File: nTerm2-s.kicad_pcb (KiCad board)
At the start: 2 copper layers, 147.3 x 55.9 mm, 107 parts, among them J1 VGA, J2 Keyboard, J3 Mouse, J4 Speaker, J5 DE9_Plug_MountingHoles, J6 USB_C_Receptacle_USB2.0_16P, K1 IM41 3V, K2 IM41 3V, K3 IM41 3V, Q1 BC817, Q2 BC817, Q3 BC817, Q4 BC817, Q5 BC817, SW1 IO0, SW2 RESET, SW3 DEFAULTS, U1 ESP32-WROOM-32, U2 LM386, U3 MAX3232E, U4 CP2102N-Axx-xQFN28, U5 NCP1117-3.3_SOT223

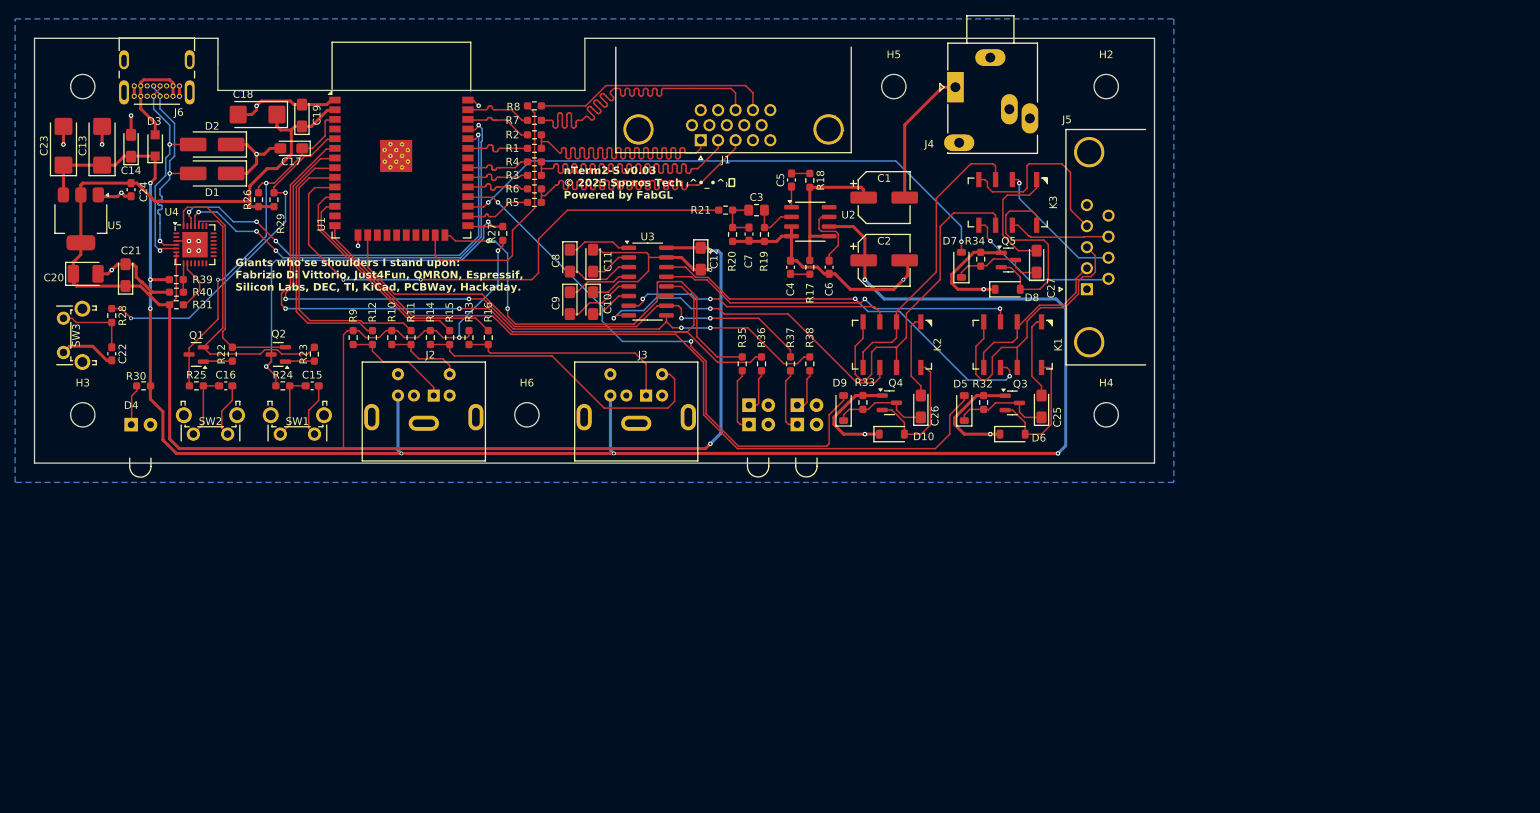
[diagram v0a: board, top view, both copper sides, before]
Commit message: More small improvements to layout.
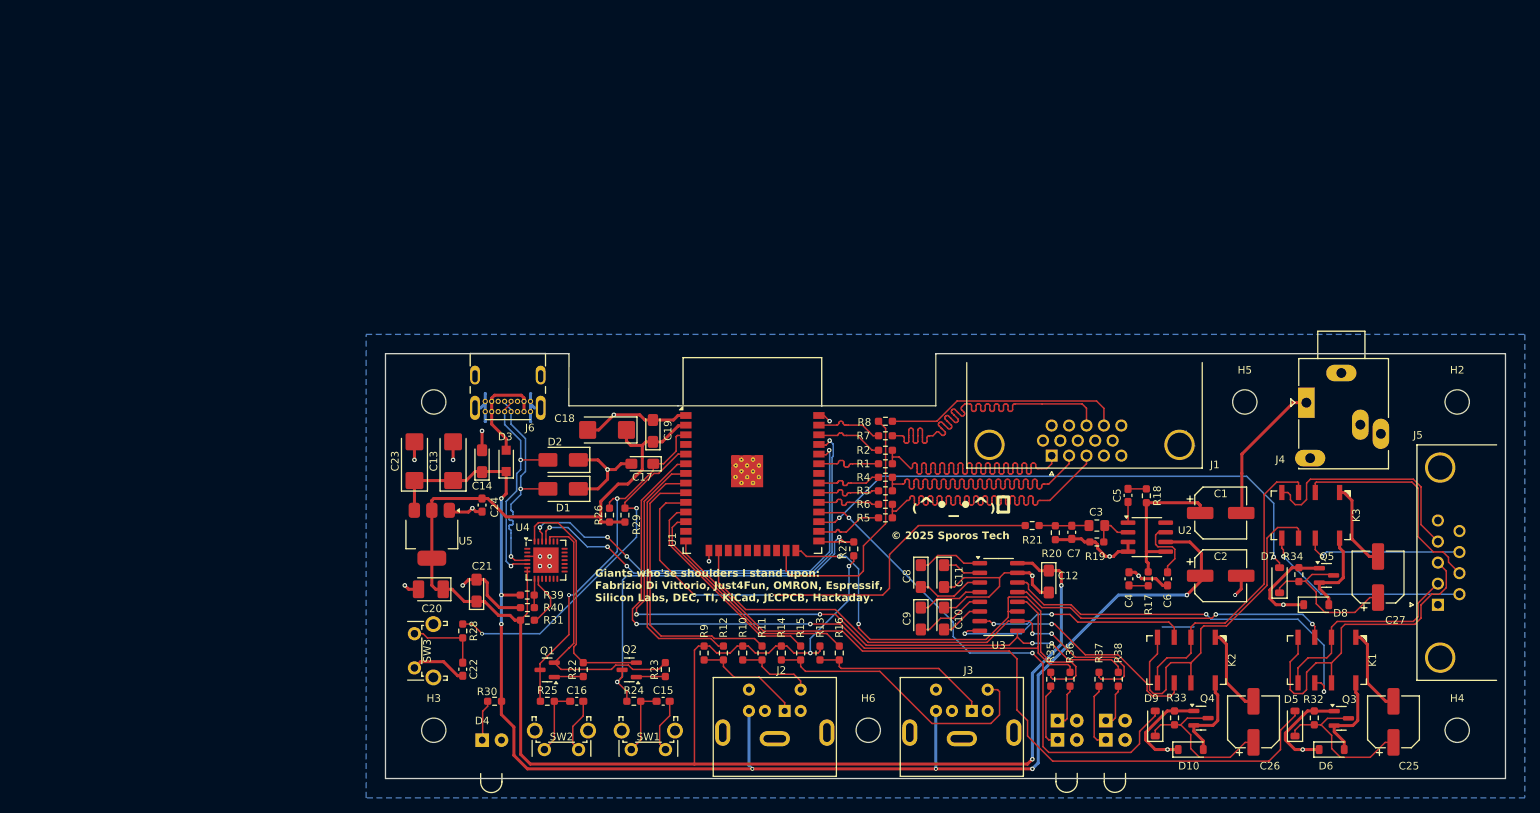
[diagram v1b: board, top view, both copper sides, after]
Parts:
- C25, C26, C27: footprint Capacitor_Tantalum_SMD:CP_EIA-3216-18_Kemet-A_Pad1.58x1.35mm_HandSolder -> Capacitor_SMD:CP_Elec_6.3x7.7
- D1, D2: footprint Diode_SMD:D_SMA_Handsoldering -> Diode_SMD:D_SMA
- K1, K2, K3: footprint Relay_SMD:Relay_2P2T_10x6mm_TE_IMxxG -> Relay_SMD:Relay_DPDT_AXICOM_IMSeries_Gullwing
- moved C12 62.4 mm to (161.4, 101.9)
- moved C25 62.2 mm to (206.7, 120.4)
- moved C10 62.1 mm to (147.6, 106.8)
- moved C9 62.1 mm to (144.5, 106.8)
- moved D1 62.1 mm to (97.5, 89.7)
- moved R1 62.1 mm to (139.9, 86.4)
- moved R15 62.1 mm to (128.7, 111.3)
- moved R4 62.1 mm to (139.9, 88.2)
- moved R6 62.1 mm to (139.9, 91.8)
- moved R8 62.1 mm to (139.9, 80.9)
- moved R9 62.1 mm to (116.0, 111.3)
- moved SW1 62.1 mm to (110.9, 124.0)
- moved C11 62.1 mm to (147.6, 101.2), turned to -90 degrees
- moved C15 62.1 mm to (110.6, 117.7)
- moved C16 62.1 mm to (99.3, 117.7)
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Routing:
- net +5V: track 249.8 -> 190.0 mm
- net RTS_OR_DTR_RLY_-: track 28.0 -> 12.2 mm
- net /_RTS: track 18.5 -> 29.3 mm, vias 1 -> 0
- net Net-(D7-K): track 12.6 -> 21.5 mm
- net Net-(D9-K): track 12.9 -> 21.6 mm
- net Net-(D5-K): track 13.1 -> 21.6 mm
- net /CTS: track 44.5 -> 36.1 mm
- net RXD_2: track 101.2 -> 93.2 mm
- net /_CTS: track 13.4 -> 21.4 mm, vias 0 -> 1
- net /RTS: track 36.1 -> 28.3 mm
- net +3V3: track 257.1 -> 250.0 mm
- net /_DSR: track 20.9 -> 27.9 mm
- net AUDIO_PWM: track 72.7 -> 66.9 mm
- net CTS_2: track 96.7 -> 90.9 mm
- net /_DTR: track 24.8 -> 30.5 mm
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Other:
- board text added: "Giants who'se shoulders I stand upon: Fabrizio Di Vittorio, Just4Fun, OMRON, Espressif, Silicon Labs, DEC, TI, KiCad, JLCPCB, Hackaday."
- board text added: "© 2025 Sporos Tech"
- board text added: "₍^•_•^₎ﾉ"
- board text removed: "Giants who'se shoulders I stand upon: Fabrizio Di Vittorio, Just4Fun, OMRON, Espressif, Silicon Labs, DEC, TI, KiCad, PCBWay, Hackaday."
- board text removed: "nTerm2-S v0.03 © 2025 Sporos Tech ₍^•_•^₎ﾉ Powered by FabGL"
